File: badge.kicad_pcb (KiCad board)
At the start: 2 copper layers, 151.5 x 81.5 mm, 52 parts, among them J1 Micro_SD_Card, J2 Conn_01x40, J3 Conn_01x40, SW1 SW_Push, SW10 SW_Push, SW11 SW_Push, SW12 SW_Push, SW13 SW_Push, SW14 SW_Push, SW15 SW_Push, SW16 SW_Push, SW17 SW_Push, SW18 SW_Push, SW19 SW_Push, SW2 SW_Push, SW20 SW_Push, SW21 SW_Push, SW22 SW_Push, SW23 SW_Push, SW24 SW_Push, SW25 SW_Push, SW26 SW_Push, SW27 SW_Push, SW28 SW_Push, SW29 SW_Push, SW3 SW_Push, SW30 SW_Push, SW31 SW_Push, SW32 SW_Push, SW33 SW_Push, SW34 SW_Push, SW35 SW_Push, SW36 SW_Push, SW37 SW_Push, SW38 SW_Push, SW39 SW_Push, SW4 SW_Push, SW40 SW_Push, SW5 SW_Push, SW6 SW_Push, SW7 SW_Push, SW8 SW_Push, SW9 SW_Push, U1 ESP32-S3-WROOM-1

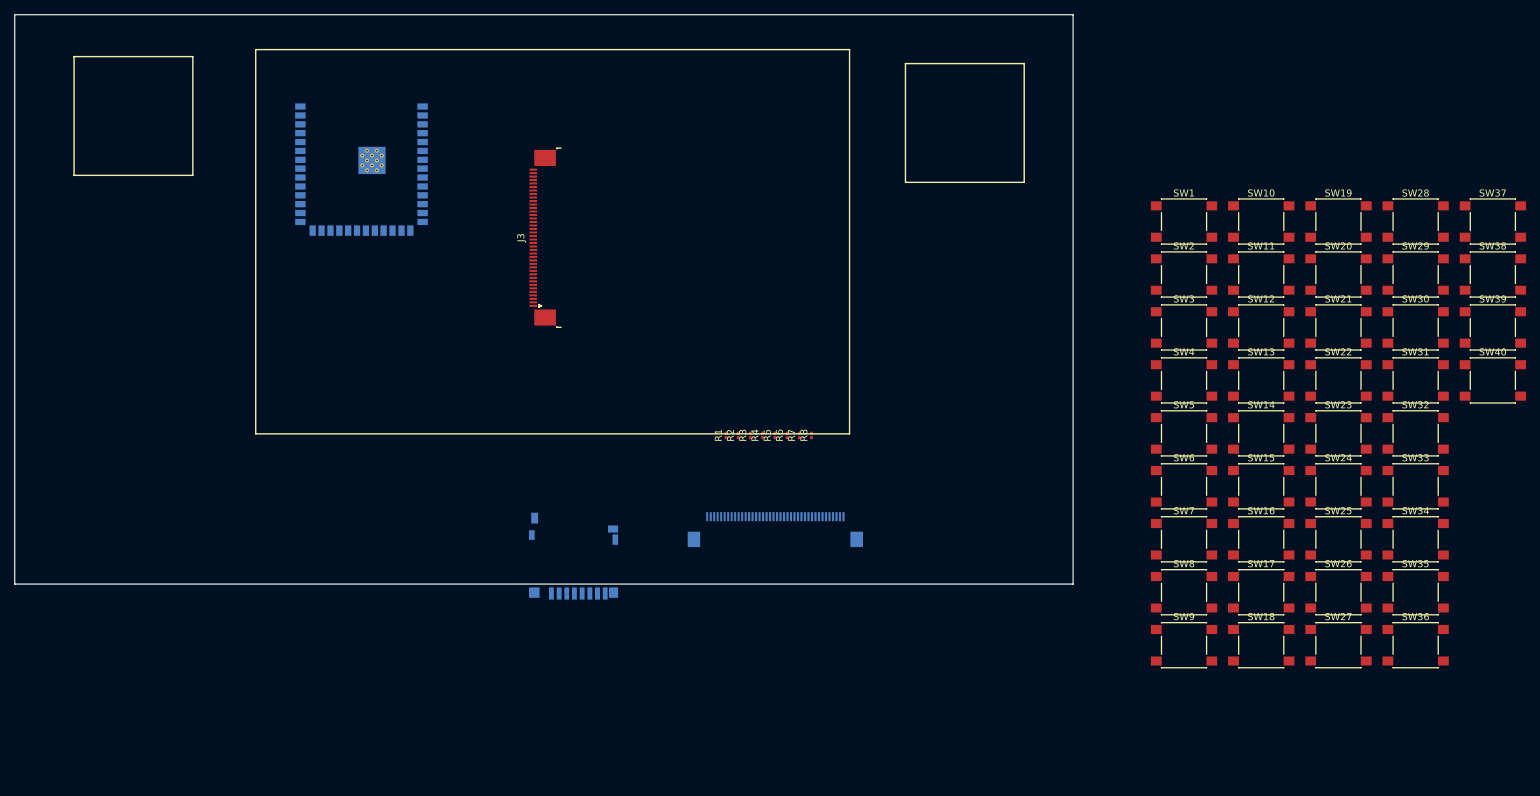
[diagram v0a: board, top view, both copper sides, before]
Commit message: upd
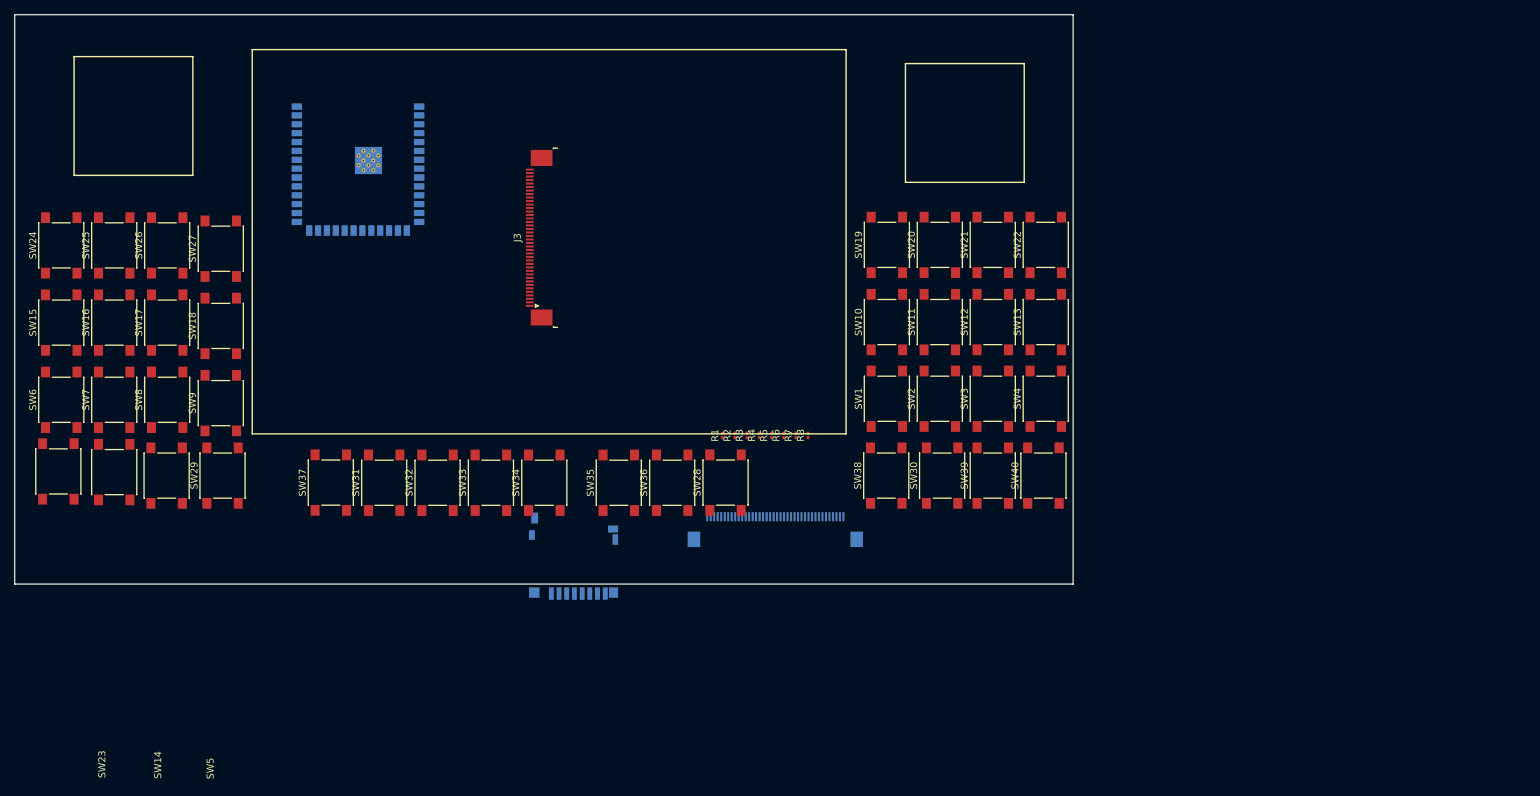
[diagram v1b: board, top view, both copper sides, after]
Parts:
- moved SW24 186.0 mm to (58.2, 65.0), turned to 90 degrees
- moved SW23 183.3 mm to (57.8, 97.4), turned to 90 degrees
- moved SW25 180.2 mm to (65.8, 65.0), turned to 90 degrees
- moved SW26 174.8 mm to (73.3, 65.0), turned to 90 degrees
- moved SW15 173.3 mm to (58.2, 76.1), turned to 90 degrees
- moved SW29 173.2 mm to (81.2, 98.0), turned to 90 degrees
- moved SW37 170.5 mm to (96.8, 99.0), turned to 90 degrees
- moved SW27 169.7 mm to (81.0, 65.5), turned to 90 degrees
- moved SW16 167.1 mm to (65.8, 76.1), turned to 90 degrees
- moved SW14 164.3 mm to (65.8, 97.5), turned to 90 degrees
- moved SW17 161.3 mm to (73.3, 76.1), turned to 90 degrees
- moved SW6 161.2 mm to (58.2, 87.1), turned to 90 degrees
- moved SW18 155.8 mm to (81.0, 76.5), turned to 90 degrees
- moved SW7 154.4 mm to (65.8, 87.1), turned to 90 degrees
- moved SW31 148.4 mm to (104.4, 99.0), turned to 90 degrees
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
